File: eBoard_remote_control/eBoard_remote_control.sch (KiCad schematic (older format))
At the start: 54 parts, among them J1 SWDIO_conn, J2 105450-0101, U1 MDBT42, U2 AP2112(3.3V), U3 MCP73831T-2ACI/OT, U4 CP2104, U5 AH49ENTR-G1, U6 AH49ENTR-G1, U7 AH49ENTR-G1, U8 SSD1306, X1 JSTPH, X2 JSTPH, X4 32.768

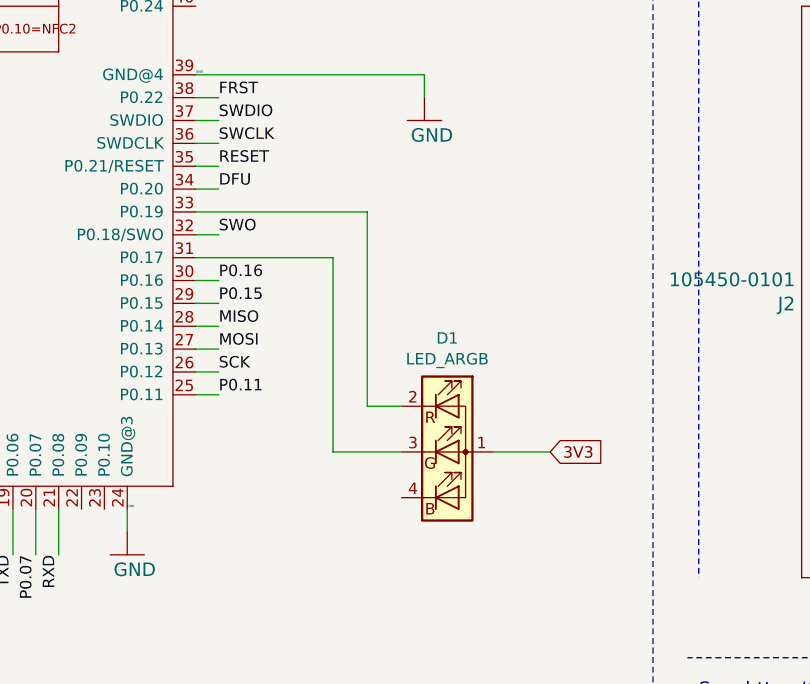
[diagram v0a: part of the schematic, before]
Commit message: V3
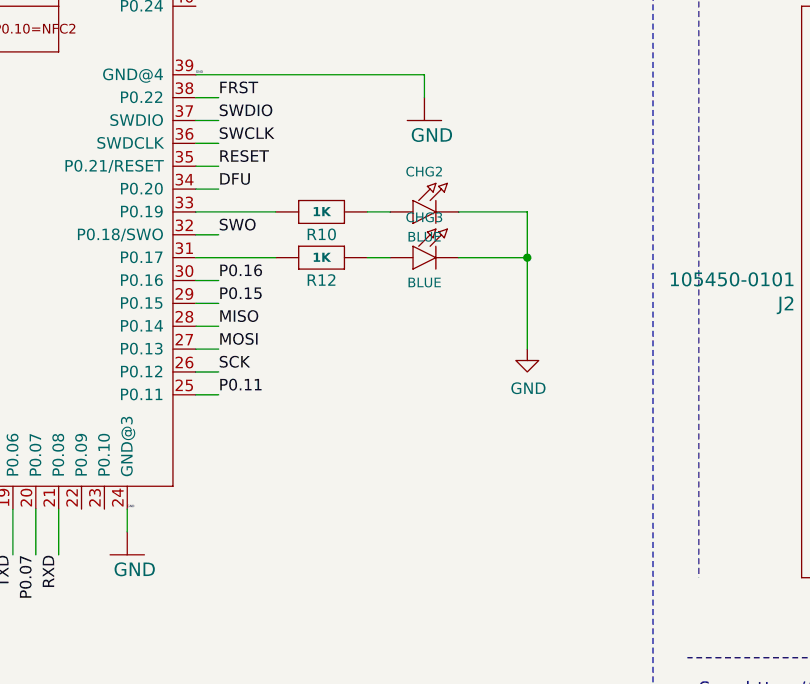
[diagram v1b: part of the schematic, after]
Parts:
- removed D1: LED_ARGB, LED_SMD:LED_Avago_PLCC4_3.2x2.8mm_CW, symbol Device:LED_ARGB
- added CHG2, CHG3: BLUE, eBoard_remote_control:CHIPLED_0805_NOOUTLINE, symbol eBoard_remote_control-eagle-import:LED0805_NOOUTLINE
- added R10, R12: 1K, eBoard_remote_control:0603-NO, symbol eBoard_remote_control-eagle-import:RESISTOR_0603_NOOUT
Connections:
- net GND: now also CHG2.C, CHG3.C
- net at U1.33 (P0.19): now also R10.2
- net at U1.31 (P0.17): now also R12.2
- new net: CHG3.A, R12.1
- new net: CHG2.A, R10.1
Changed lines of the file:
@@
 	9600 3550 9600 3800
 Connection ~ 9600 3550
+Wire Wire Line
+	5750 7700 5650 7700
 $Comp
-L Device:LED_ARGB D1
-U 1 1 5CCBD6F3
-P 6000 8550
-F 0 "D1" H 6000 9047 50  0000 C CNN
-F 1 "LED_ARGB" H 6000 8956 50  0000 C CNN
-F 2 "LED_SMD:LED_Avago_PLCC4_3.2x2.8mm_CW" H 6000 8500 50  0001 C CNN
-F 3 "~" H 6000 8500 50  0001 C CNN
-	1    6000 8550
+L eBoard_remote_control-eagle-import:LED0805_NOOUTLINE CHG3
+U 1 0 5CC2A068
+P 5950 7700
+F 0 "CHG3" H 5900 7875 42  0000 C CNN
+F 1 "BLUE" H 5900 7590 42  0000 C CNN
+F 2 "eBoard_remote_control:CHIPLED_0805_NOOUTLINE" H 5950 7700 50  0001 C CNN
+F 3 "" H 5950 7700 50  0001 C CNN
+	1    5950 7700
+	1    0    0    -1
+$EndComp
+$Comp
+L eBoard_remote_control-eagle-import:RESISTOR_0603_NOOUT R12
+U 1 0 5CC2A06E
+P 5450 7700
+F 0 "R12" H 5450 7800 50  0000 C CNN
+F 1 "1K" H 5450 7700 40  0000 C CNB
+F 2 "eBoard_remote_control:0603-NO" H 5450 7700 50  0001 C CNN
+F 3 "" H 5450 7700 50  0001 C CNN
+	1    5450 7700
+	-1   0    0    1
+$EndComp
+Wire Wire Line
+	5750 7500 5650 7500
+$Comp
+L eBoard_remote_control-eagle-import:LED0805_NOOUTLINE CHG2
+U 1 0 5CC59875
+P 5950 7500
+F 0 "CHG2" H 5900 7675 42  0000 C CNN
+F 1 "BLUE" H 5900 7390 42  0000 C CNN
+F 2 "eBoard_remote_control:CHIPLED_0805_NOOUTLINE" H 5950 7500 50  0001 C CNN
+F 3 "" H 5950 7500 50  0001 C CNN
+	1    5950 7500
+	1    0    0    -1
+$EndComp
+$Comp
+L eBoard_remote_control-eagle-import:RESISTOR_0603_NOOUT R10
+U 1 0 5CC5987B
+P 5450 7500
+F 0 "R10" H 5450 7600 50  0000 C CNN
+F 1 "1K" H 5450 7500 40  0000 C CNB
+F 2 "eBoard_remote_control:0603-NO" H 5450 7500 50  0001 C CNN
+F 3 "" H 5450 7500 50  0001 C CNN
+	1    5450 7500
+	-1   0    0    1
+$EndComp
+Wire Wire Line
+	5250 7500 4900 7500
+Wire Wire Line
+	5250 7700 4900 7700
+Wire Wire Line
+	6050 7500 6350 7500
+Wire Wire Line
+	6350 7500 6350 7700
+Wire Wire Line
+	6350 7700 6050 7700
+Connection ~ 6350 7700
+$Comp
+L power:GND #PWR0105
+U 1 1 5CCD9F47
+P 6350 8100
+F 0 "#PWR0105" H 6350 7850 50  0001 C CNN
+F 1 "GND" H 6355 7927 50  0000 C CNN
+F 2 "" H 6350 8100 50  0001 C CNN
+F 3 "" H 6350 8100 50  0001 C CNN
+	1    6350 8100
 	1    0    0    -1
 $EndComp
 Wire Wire Line
-	4900 7700 5500 7700
-Wire Wire Line
-	5500 7700 5500 8550
-Wire Wire Line
-	5500 8550 5800 8550
-Wire Wire Line
-	5800 8350 5650 8350
-Wire Wire Line
-	5650 8350 5650 7500
-Wire Wire Line
-	5650 7500 4900 7500
-Wire Wire Line
-	6450 8550 6200 8550
-Text GLabel 6450 8550 2    50   Input ~ 0
-3V3
+	6350 7700 6350 8100
 $EndSCHEMATC
